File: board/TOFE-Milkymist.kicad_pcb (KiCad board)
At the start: 2 copper layers, 1 part

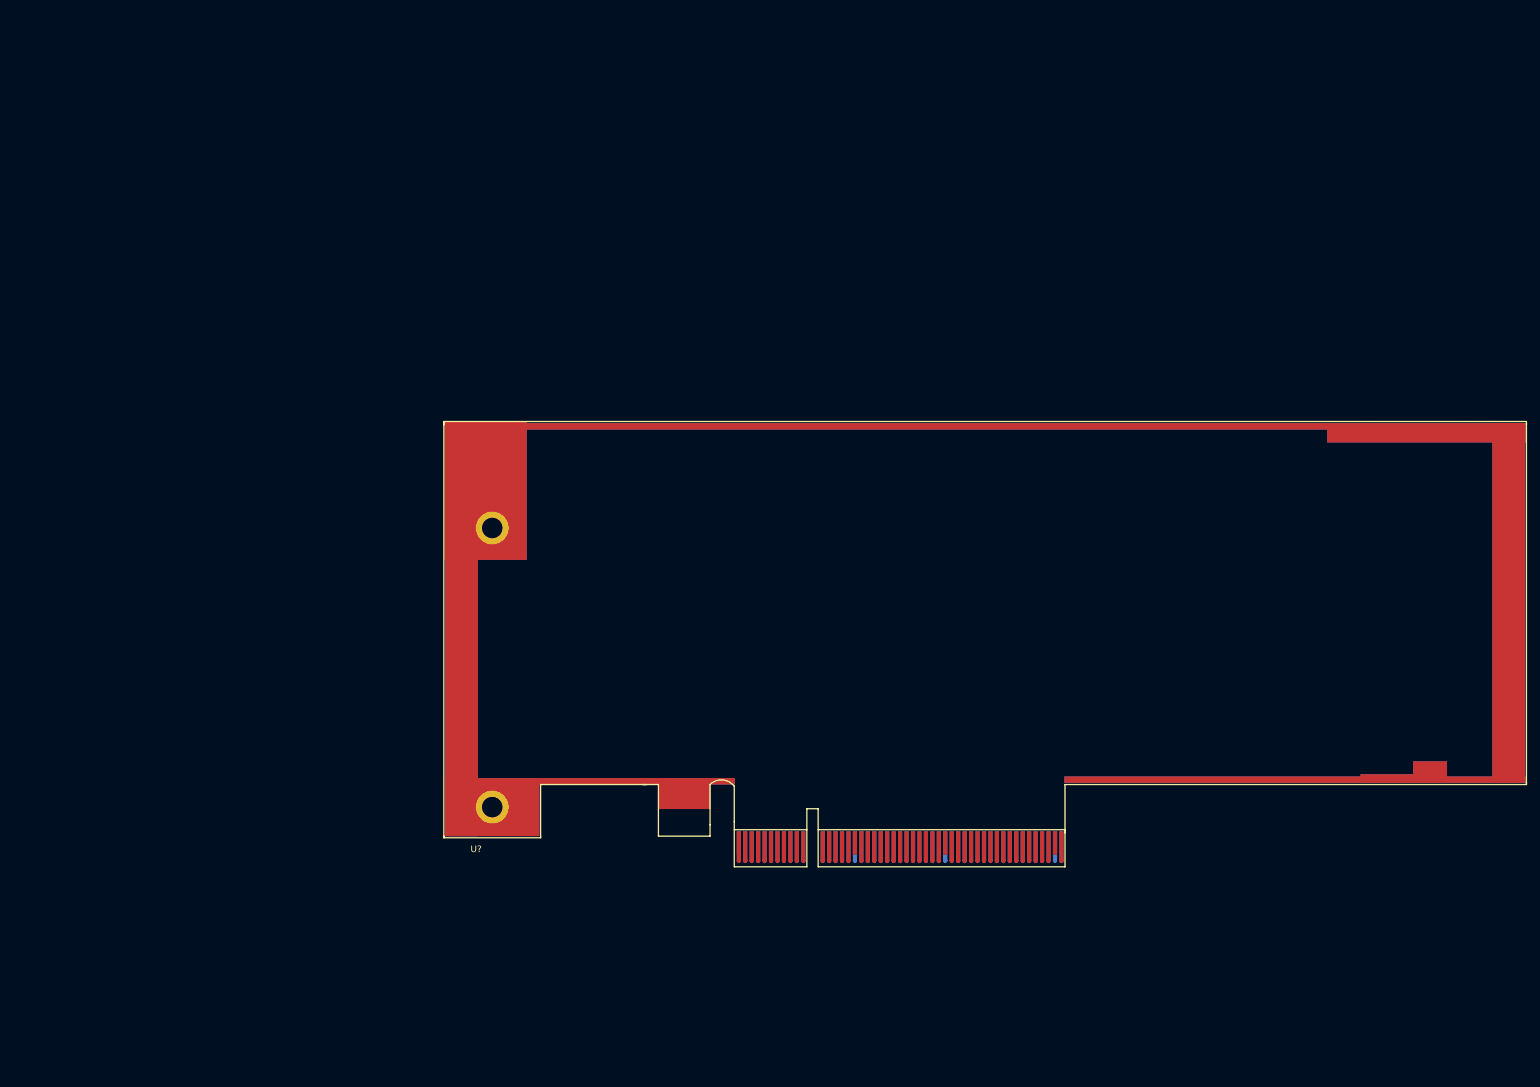
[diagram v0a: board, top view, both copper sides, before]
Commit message: Creating TOFE-Milkymist!
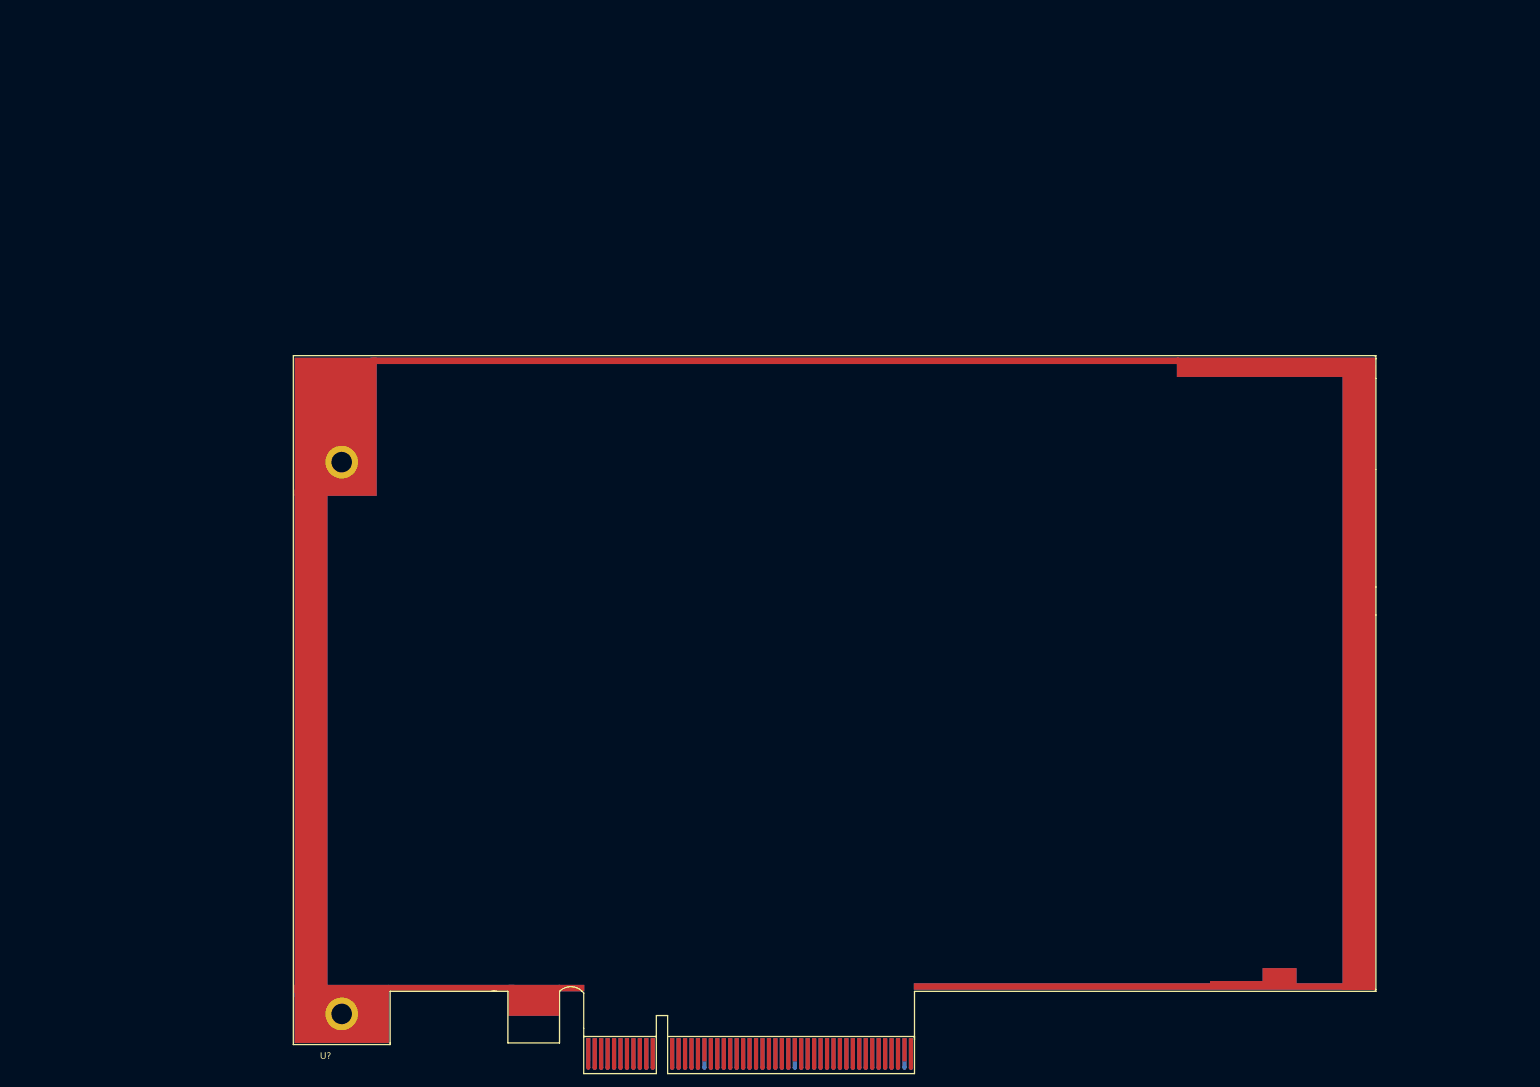
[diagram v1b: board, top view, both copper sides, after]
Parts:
- removed the U? at (148.4, 164.6)
- added U?: TOFE_Milkymist_Expansion_Board_8x_FullHeight, TOFE_8X_FullHeight, F.Cu at (125.1, 196.7)

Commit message: Initial version from on 2015-11-03
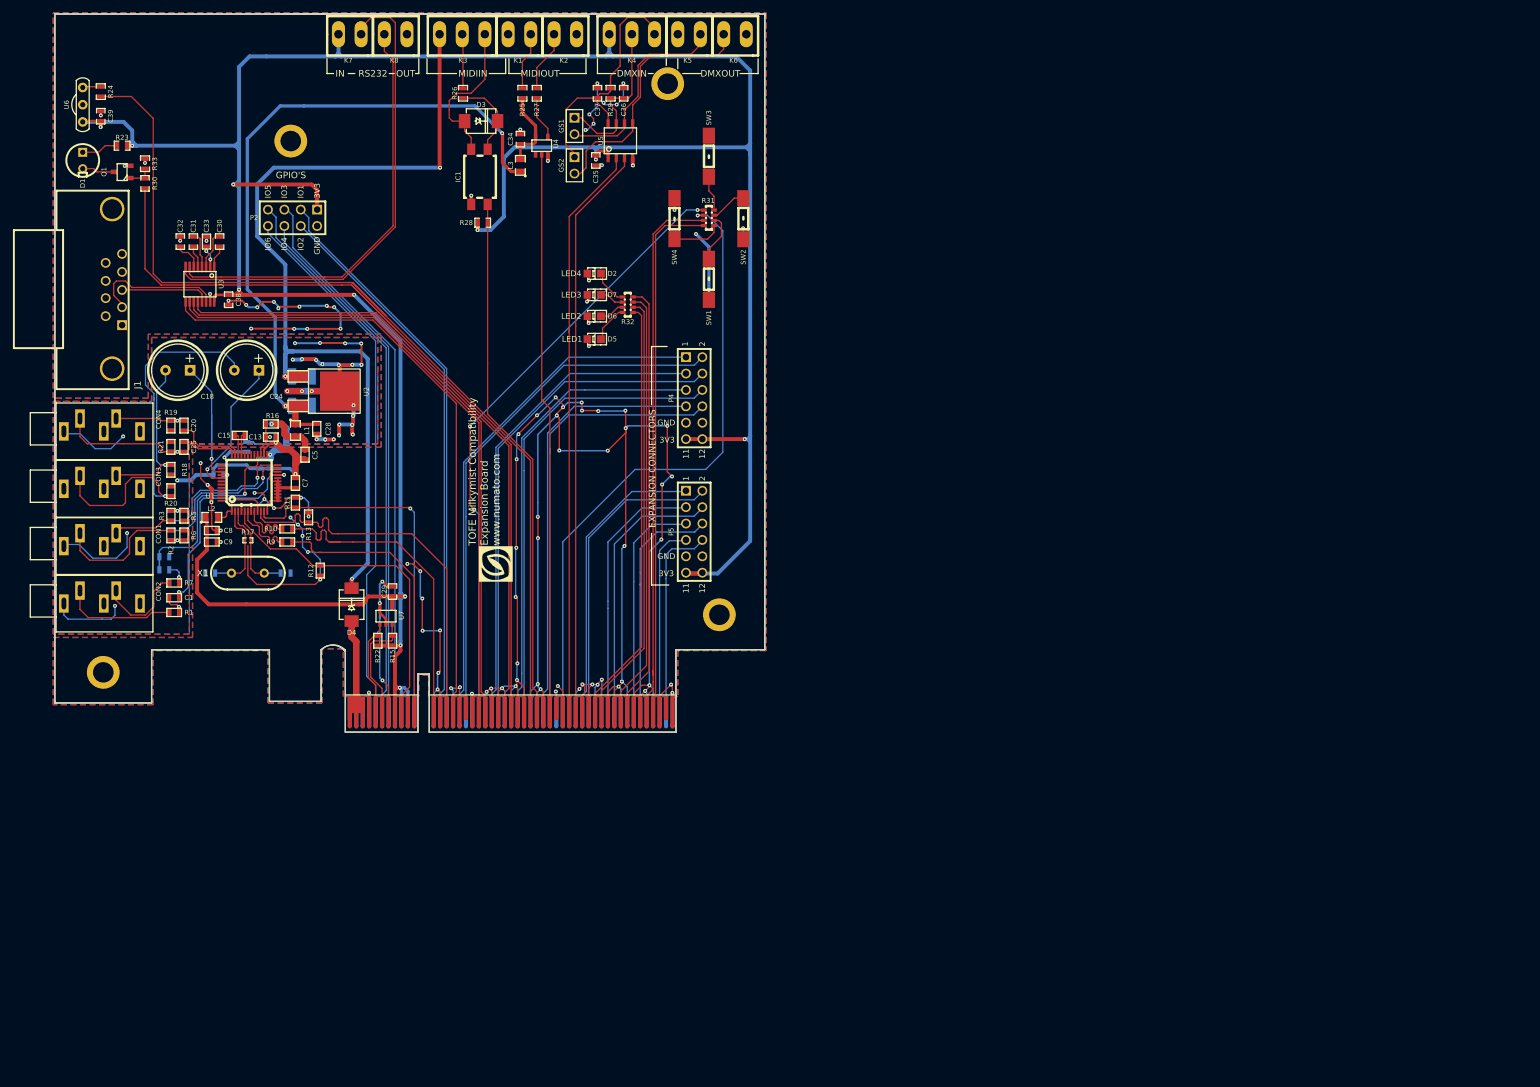
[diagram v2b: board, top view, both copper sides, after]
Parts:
- removed U?: TOFE_Milkymist_Expansion_Board_8x_FullHeight, TOFE_8X_FullHeight
- added 1PIN: P***, MH-4MM, F.Cu at (180.8, 64.5)
- added 1PIN: P***, MH-4MM, F.Cu at (181.1, 52.8)
- added C1: 1uF, SM0603, F.Cu at (106.6, 127.4)
- added C10: 100uF, SM1210, B.Cu at (126.4, 93.2)
- added C11: 0.1uF, SM0603, B.Cu at (121.5, 106.7)
- added C12: 1uF, SM0603, B.Cu at (119.9, 106.7)
- added C13: 0.1uF, SM0603, F.Cu at (121.6, 102.6)
- added C14: 3.3uF, SM0603, B.Cu at (121.6, 102.6)
- added C15: 22nF, SM0603, F.Cu at (116.8, 102.3)
- added C16: 1uF, SM0603, B.Cu at (113.5, 108.4)
- added C17: 100uF, SM1210, B.Cu at (126.4, 97.7)
- added C18: 220uF, C_Electrolytic, F.Cu at (107.2, 92.2)
- added C19: 20pF, SM0603, B.Cu at (123.9, 123.6)
- added C2: 1uF, SM0603, B.Cu at (106.1, 117.8)
- added C20: 1uF, SM0603, F.Cu at (108.1, 100.8)
- added C21: 220pF, SM0603, B.Cu at (106.1, 107.6)
- added C22: 220pF, SM0603, B.Cu at (106.1, 100.8)
- added C23: 20pF, SM0603, B.Cu at (112.2, 123.6)
- added C24: 220uF, C_Electrolytic, F.Cu at (117.9, 92.2)
- added C25: 1uF, SM0603, F.Cu at (108.1, 104.1)
- added C26: 220pF, SM0603, B.Cu at (106.1, 110.9)
- added C27: 220pF, SM0603, B.Cu at (106.1, 104.1)
- added C28: 0.1uF, SM0603, F.Cu at (128.7, 101.3)
- added C29: 0.1uF, SM0603_Capa, F.Cu at (140.5, 126.5)
- added C3: 1uF, SM0603, B.Cu at (106.1, 114.7)
- added C30: 0.1uF, SM0603_Capa, F.Cu at (113.7, 72.3)
- added C31: 0.1uF, SM0603_Capa, F.Cu at (109.6, 72.3)
- added C32: 0.1uF, SM0603_Capa, F.Cu at (107.6, 72.3)
- added C33: 0.1uF, SM0603, F.Cu at (111.6, 72.3)
- added C34: 0.1uF, SM0603_Capa_new, F.Cu at (160.3, 56.4)
- added C35: 0.1uF, SM0603_Capa_new, F.Cu at (172.0, 59.7)
- added C36: 15pF, SM0603_Capa, F.Cu at (176.3, 49.3)
- added C37: 15pF, SM0603_Capa, F.Cu at (172.2, 49.3)
- added C38: 0.1uF, SM0603_Capa_new, F.Cu at (115.1, 81.3)
- added C39: 10uF, SM0603_Capa_new, F.Cu at (95.2, 52.8)
- added C4: 220pF, SM0603, B.Cu at (106.6, 125.2)
- added C5: 0.1uF, SM0603, F.Cu at (126.9, 105.3)
- added C6: 2.2uF, SM0603, B.Cu at (105.1, 121.1)
- added C7: 0.1uF, SM0603, F.Cu at (125.4, 109.7)
- added C8: 0.1uF, SM0603, F.Cu at (112.5, 117.0)
- added C9: 1uF, SM0603, F.Cu at (112.5, 118.8)
- added CON1: AUDIO_JACK_3535NG, 3.5MM_Stereo_Jack_Socket, F.Cu at (88.3, 118.6)
- added CON2: AUDIO_JACK_3535NG, 3.5MM_Stereo_Jack_Socket, F.Cu at (88.3, 127.4)
- added CON3: AUDIO_JACK_3535NG, 3.5MM_Stereo_Jack_Socket, F.Cu at (88.3, 109.7)
- added CON4: AUDIO_JACK_3535NG, 3.5MM_Stereo_Jack_Socket, F.Cu at (88.3, 100.8)
- added D1: IR-LED, LEDV, F.Cu at (92.5, 59.7)
- added D2: LED, LED-0805-New, F.Cu at (171.7, 77.2)
- added D3: DIODE, DO214AA, F.Cu at (154.2, 53.6)
- added D4: DIODE, DO214AA, F.Cu at (134.1, 128.5)
- added D5: LED, LED-0805-New, F.Cu at (171.7, 87.4)
- added D6: LED, LED-0805-New, F.Cu at (171.7, 83.8)
- added D7: LED, LED-0805-New, F.Cu at (171.7, 80.5)
- added G***: LOGO, LOGO, F.Cu at (156.5, 122.2)
- added GS1: GS2, PIN_ARRAY_2X1, F.Cu at (168.7, 54.4)
- added GS2: GS2, PIN_ARRAY_2X1, F.Cu at (168.7, 60.5)
- added IC1: PC817, SMD_PC817, F.Cu at (153.9, 62.2)
- added J1: DB9, DB9_Female, F.Cu at (97.3, 79.8)
- added K1: CONN_2, ScrewTerm2_138MIL, F.Cu at (158.4, 40.1)
- added K2: CONN_2, ScrewTerm2_138MIL, F.Cu at (165.5, 40.1)
- added K3: CONN_3, ScrewTerm3_138MIL, F.Cu at (151.3, 40.1)
- added K4: CONN_3, ScrewTerm3_138MIL, F.Cu at (177.5, 40.1)
- added K5: CONN_2, ScrewTerm2_138MIL, F.Cu at (184.7, 40.1)
- added K6: CONN_2, ScrewTerm2_138MIL, F.Cu at (191.8, 40.1)
- added K7: CONN_2, ScrewTerm2_138MIL, F.Cu at (132.1, 40.1)
- added K8: CONN_2, ScrewTerm2_138MIL, F.Cu at (139.2, 40.1)
- added L1: 4.7uH, SM0805, F.Cu at (125.4, 101.5)
- added L2: 4.7uH, SM0805, F.Cu at (112.5, 115.0)
- added L3: 4.7uH, SM0805, F.Cu at (160.3, 60.5)
- added P2: CONN_4X2, pin_array_4x2, F.Cu at (125.0, 68.6)
- added P4: CONN_6X2, pin_array_6x2, F.Cu at (187.2, 96.5)
- added P5: CONN_6X2, pin_array_6x2, F.Cu at (187.2, 117.2)
- added Q1: TRANSISTOR-NPN, SOT23-TRANSISTOR-NPN, F.Cu at (98.6, 61.5)
- added R1: 1K, SM0603, F.Cu at (106.6, 129.7)
- added R10: 27.4, SM0603, F.Cu at (124.1, 116.8)
- added R11: 4.75K, SM0603, F.Cu at (125.4, 112.7)
- added R12: 4.75K, SM0603, F.Cu at (129.3, 123.2)
- added R13: 4.75K, SM0603, F.Cu at (127.4, 115.0)
- added R14: 0R, SM0603, B.Cu at (117.9, 104.1)
- added R15: 10K, SM0603, F.Cu at (140.5, 134.1)
- added R16: R, SM0603, F.Cu at (121.6, 100.5)
- added R17: 1M, SM0402, F.Cu at (118.0, 118.6)
- added R18: 10K, SM0603, F.Cu at (106.1, 107.6)
- added R19: 10K, SM0603, F.Cu at (106.1, 100.8)
- added R2: 6.81K, SM0603, F.Cu at (106.1, 117.8)
- added R20: 10K, SM0603, F.Cu at (106.1, 110.9)
- added R21: 10K, SM0603, F.Cu at (106.1, 104.1)
- added R22: 10K, SM0603, F.Cu at (138.2, 134.1)
- added R23: 47R, SM0603_Resistor_new, F.Cu at (98.6, 57.4)
- added R24: 1K, SM0603_Resistor_new, F.Cu at (95.2, 49.0)
- added R25: 220R, SM0603_Resistor_new, F.Cu at (160.6, 49.3)
- added R26: 220R, SM0603_Resistor_new, F.Cu at (151.4, 49.3)
- added R27: 220R, SM0603_Resistor_new, F.Cu at (162.8, 49.3)
- added R28: 220R, SM0603_Resistor_new, F.Cu at (154.4, 69.3)
- added R29: 60R, SM0603_Resistor_new, F.Cu at (174.2, 49.3)
- added R3: 6.81K, SM0603, F.Cu at (106.1, 114.7)
- added R30: 2K2, SM0603_Capa_new, F.Cu at (102.1, 63.2)
- added R31: 680R, RES_NET4, F.Cu at (189.5, 68.6)
- added R32: 10K, RES_NET4, F.Cu at (176.9, 82.0)
- added R33: 10K, SM0603_Resistor_new, F.Cu at (102.1, 60.2)
- added R4: 47K, SM0603, B.Cu at (106.6, 129.7)
- added R5: 6.81K, SM0603, F.Cu at (108.1, 114.7)
- added R6: 6.81K, SM0603, F.Cu at (108.1, 117.8)
- added R7: 47R, SM0603, F.Cu at (106.6, 125.2)
- added R8: 2.2K, SM0603, B.Cu at (105.1, 123.1)
- added R9: 27.4, SM0603, F.Cu at (124.1, 118.8)
- added SW1: SW_PUSH, Switch_SMD_new, F.Cu at (189.5, 78.0)
- added SW2: SW_PUSH, Switch_SMD_new, F.Cu at (194.8, 68.6)
- added SW3: SW_PUSH, Switch_SMD_new, F.Cu at (189.5, 59.2)
- added SW4: SW_PUSH, Switch_SMD_new, F.Cu at (184.2, 68.8)
- added U1: LM4550, LQFP48, F.Cu at (118.3, 109.7)
- added U2: 7805_N, DPAK2, F.Cu at (125.9, 95.4)
- added U3: ST3232CDR, ssop-16, F.Cu at (110.6, 78.9)
- added U4: SN74LVC1G17, SOT23-5_SN74LVC1G17DBVR, F.Cu at (163.6, 57.4)
- added U5: ISL83490, SOIC-8_ISL83490, F.Cu at (175.8, 56.6)
- added U6: IR-RX, IR_REC_TH, F.Cu at (92.5, 51.1)
- added U7: 24AA01/24LC01B, SOT23-5_24AA01, F.Cu at (139.4, 130.3)
- added U8: TIMVIDEOS-PCIE-8X, NumatoOpsis_PCIe_8X_HL_NW_110x110, F.Cu at (88.1, 143.8)
- added X1: CRYSTAL, HC-49V, F.Cu at (118.0, 123.6)
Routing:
- net /GND: track 0.00 -> 568.0 mm, vias 0 -> 113
- net /VCC3V3: track 0.00 -> 492.0 mm, vias 0 -> 11
- net /IR_OUT: track 0.00 -> 151.0 mm
- net /VCC12V: track 0.00 -> 141.5 mm, vias 0 -> 3
- net /IR_EN: track 0.00 -> 131.8 mm
- net /AGND: track 0.00 -> 130.0 mm, vias 0 -> 29
- net /VCC5V0: track 0.00 -> 104.4 mm, vias 0 -> 2
- net /RS232-RX1: track 0.00 -> 99.6 mm
- net /RS232-TX1: track 0.00 -> 98.2 mm
- net /RS232-TX2: track 0.00 -> 98.1 mm
- net /RS232-RX2: track 0.00 -> 97.3 mm
- net /SW2: track 0.00 -> 97.0 mm, vias 0 -> 1
- net /SW1: track 0.00 -> 94.8 mm, vias 0 -> 3
- net /DMX_TX: track 0.00 -> 89.1 mm
- net /DMX_RX: track 0.00 -> 88.9 mm
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- added copper zone on B.Cu, net /AGND
- added copper zone on F.Cu, net /AGND
- added copper zone on B.Cu, net /GND
- added copper zone on F.Cu, net /GND
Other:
- board outline added: 110 x 111.3 mm
- net class Default: clearance 0.254 -> 0.1524; trace_width 0.254 -> 0.2032; via_dia 0.889 -> 0.6096; via_drill 0.635 -> 0.3048
- rule trace_clearance: 0.254 -> 0.1524
- rule trace_min: 0.254 -> 0.2032
- rule via_min_drill: 0.508 -> 0.3048
- rule via_min_size: 0.889 -> 0.6096
- board text added: "1"
- board text added: "11"
- board text added: "12"
- board text added: "2"
- board text added: "3V3"
- board text added: "DMXIN"
- board text added: "DMXOUT"
- board text added: "EXPANSION CONNECTORS"
- board text added: "GND"
- board text added: "GPIO'S"
- board text added: "HP OUT"
- board text added: "IN"
- board text added: "IO1"
- board text added: "IO2"
- board text added: "IO3"
- board text added: "IO4"
- board text added: "IO5"
- board text added: "IO6"
- board text added: "LED1"
- board text added: "LED2"
- board text added: "LED3"
- board text added: "LED4"
- board text added: "LINE IN"
- board text added: "LINE OUT"
- board text added: "MIC"
- board text added: "MIDIIN"
- board text added: "MIDIOUT"
- board text added: "OUT"
- board text added: "RS232"
- board text added: "TOFE Milkymist Compatibility Expansion Board www.numato.com"
